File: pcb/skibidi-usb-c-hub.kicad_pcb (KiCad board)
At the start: 2 copper layers, 17.5 x 39 mm, 20 parts, among them U1 CH334P

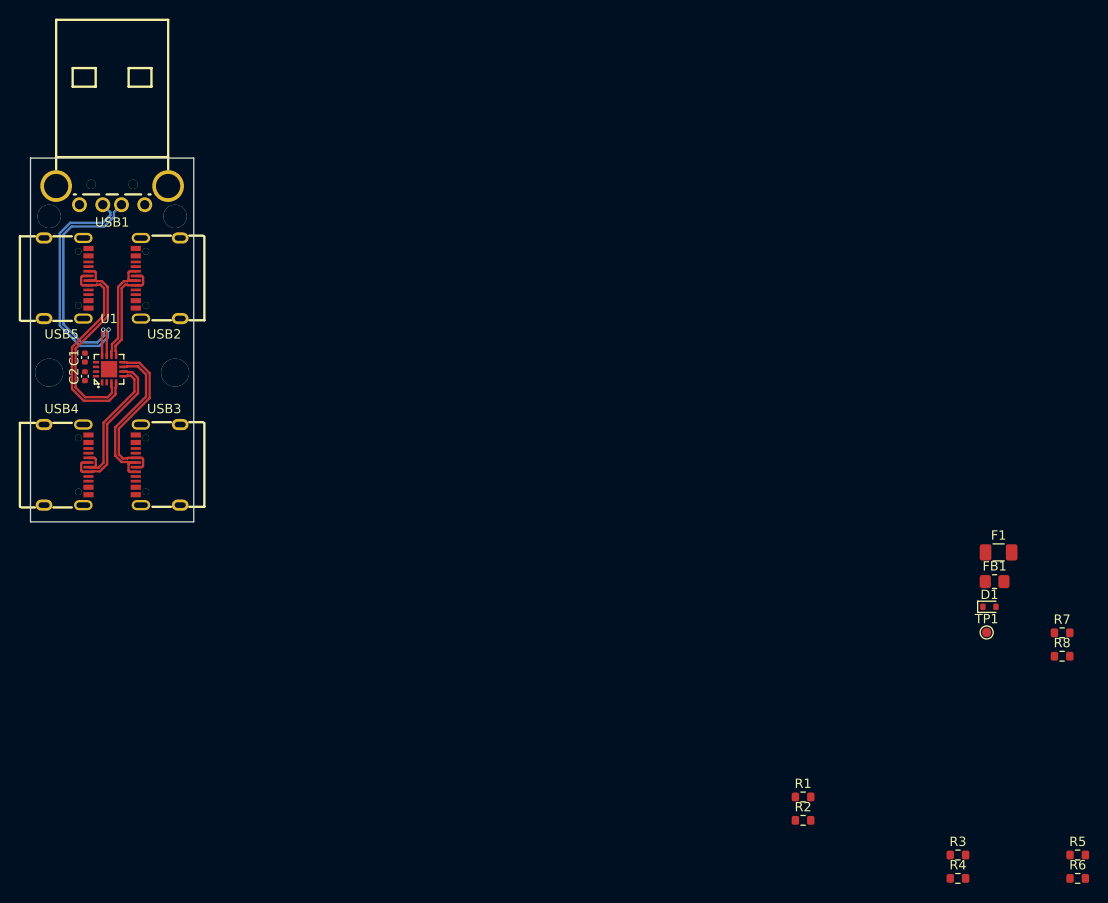
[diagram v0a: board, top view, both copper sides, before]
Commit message: finished pcb and bom, added schematic pdf, step file for pcb, and gerbers
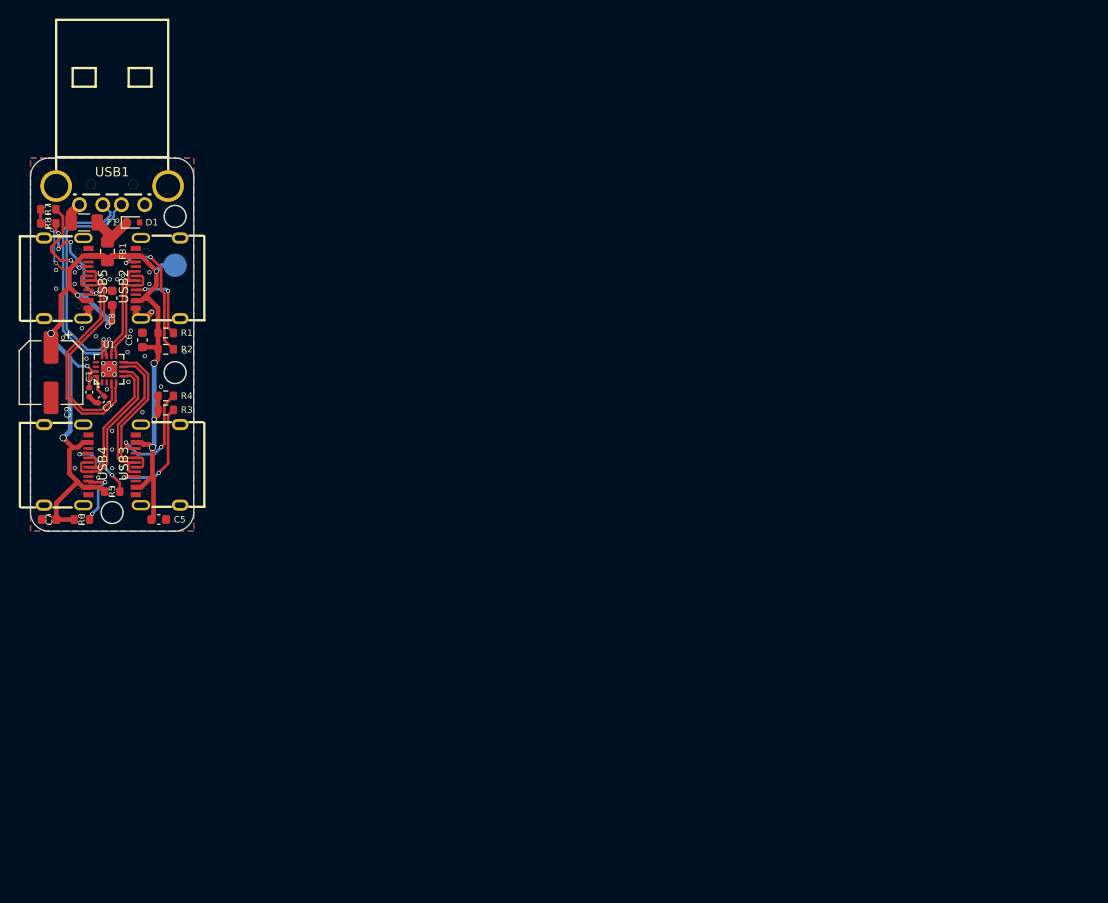
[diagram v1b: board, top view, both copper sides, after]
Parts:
- added C5: 10u, Capacitor_SMD:C_0603_1608Metric, F.Cu at (43.8, 68.8)
- added C6: 10u, Capacitor_SMD:C_0603_1608Metric, F.Cu at (42.0, 49.5)
- added C7: 10u, Capacitor_SMD:C_0603_1608Metric, F.Cu at (32.0, 68.8)
- added C8: 10u, Capacitor_SMD:C_0603_1608Metric, F.Cu at (38.8, 45.0)
- added C9: 220u, Capacitor_SMD:CP_Elec_6.3x5.8, F.Cu at (32.2, 53.0)
- C2: value 100n -> 4.7u
- TP1: footprint TestPoint:TestPoint_Pad_D1.0mm -> TestPoint:TestPoint_Pad_D2.5mm; moved to B.Cu
- moved R8 118.2 mm to (31.9, 37.0)
- moved R7 117.8 mm to (31.9, 35.5)
- moved R6 113.5 mm to (35.5, 68.8)
- moved R5 110.6 mm to (38.8, 65.8)
- moved F1 104.2 mm to (35.8, 36.9)
- moved FB1 101.5 mm to (38.2, 40.0), turned to -90 degrees
- moved D1 100.6 mm to (41.0, 36.9)
- moved R4 99.4 mm to (44.5, 55.5)
- moved R3 97.4 mm to (44.5, 57.0)
- moved TP1 95.5 mm to (45.5, 41.5)
- moved R2 85.0 mm to (44.5, 50.5)
- moved R1 84.5 mm to (44.5, 48.8)
- moved C1 3.74 mm to (36.3, 55.1), turned to -90 degrees
- moved C2 3.07 mm to (37.6, 55.9), turned to -135 degrees
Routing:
- net VBUS: track 0.00 -> 113.9 mm, vias 0 -> 11
- net Net-(USB2-CC2): track 0.00 -> 14.9 mm, vias 0 -> 2
- net Net-(USB3-CC1): track 0.00 -> 12.7 mm, vias 0 -> 2
- net Net-(USB5-CC2): track 0.00 -> 12.3 mm, vias 0 -> 4
- net Net-(USB3-CC2): track 0.00 -> 12.1 mm, vias 0 -> 2
- net Net-(USB5-CC1): track 0.00 -> 10.1 mm, vias 0 -> 2
- net Net-(USB2-CC1): track 0.00 -> 8.32 mm, vias 0 -> 2
- net Net-(USB4-CC1): track 0.00 -> 7.53 mm, vias 0 -> 2
- net Net-(USB4-CC2): track 0.00 -> 6.53 mm, vias 0 -> 2
- net Net-(D1-A1): track 0.00 -> 5.50 mm
- net GND: track 0.00 -> 5.38 mm, vias 0 -> 35
- net /USB C 4/D-: track 22.6 -> 25.3 mm
- net /USB C 4/D+: track 23.3 -> 25.9 mm
- net +3V3: track 0.00 -> 2.56 mm
- net Net-(USB1-VCC): track 0.00 -> 2.27 mm
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- added copper zone on B.Cu, net GND
- added copper zone on F.Cu, net GND
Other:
- board size 17.5 x 39 mm -> 17.5 x 40 mm
